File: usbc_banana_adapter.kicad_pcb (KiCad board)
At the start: 2 copper layers, 32 x 25 mm, 26 parts, among them P1 UJ20-C-V-C-3-SMT-TR, SW1 DSHP02TJGER, U1 TPS25810RVCR, U3 TPS2514DBVR

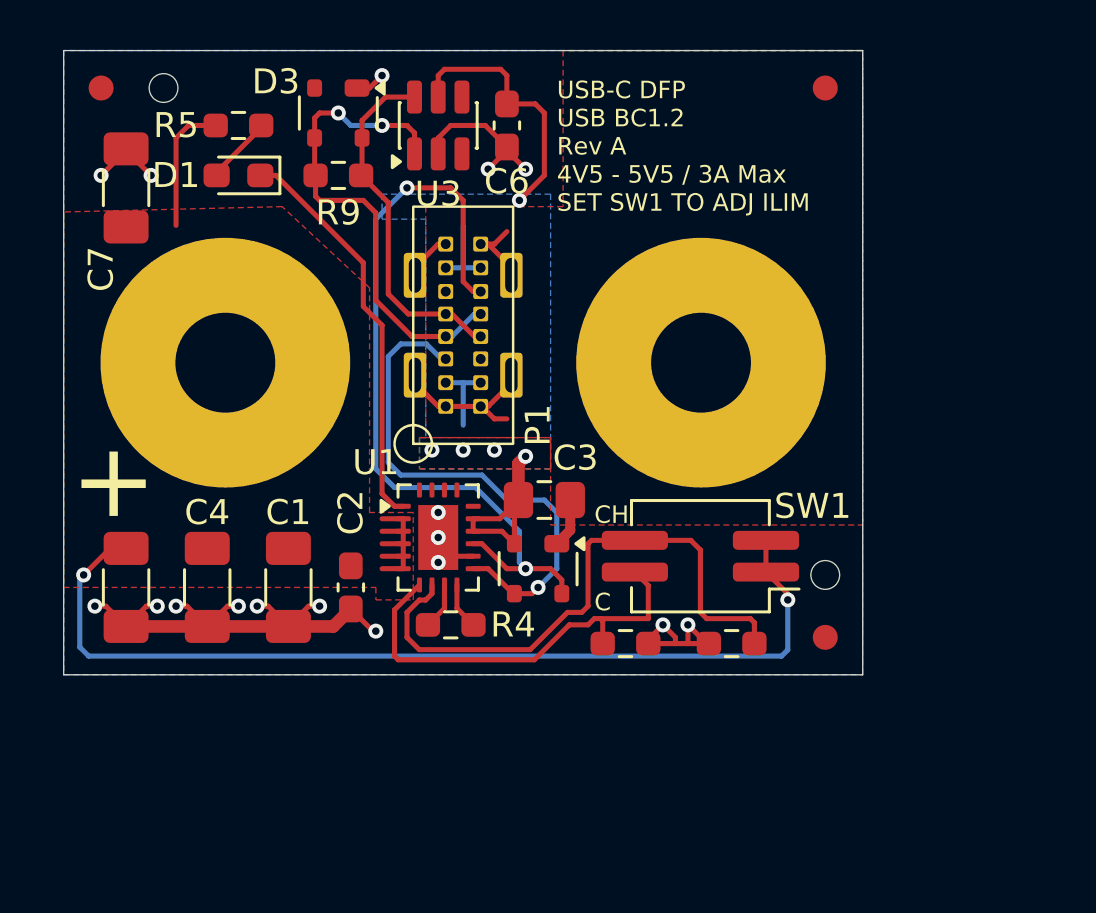
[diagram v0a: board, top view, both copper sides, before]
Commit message: swap banana
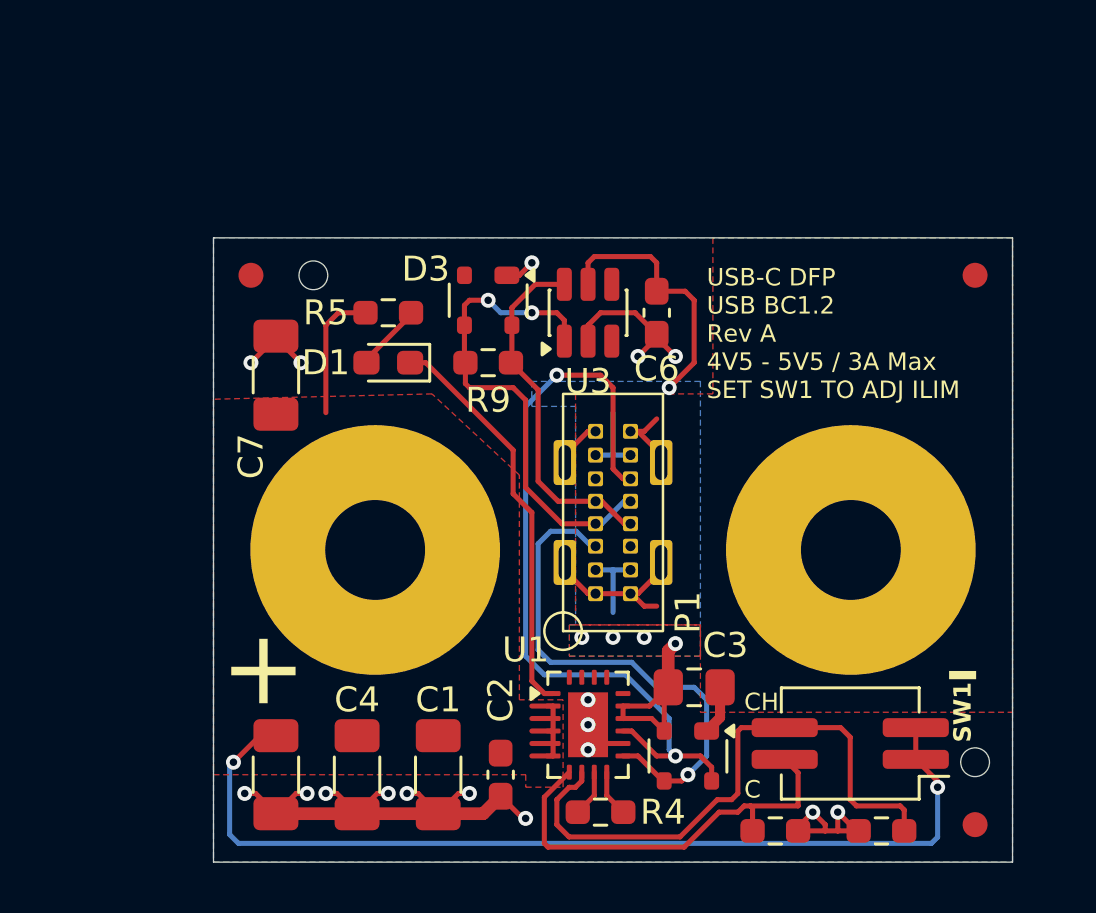
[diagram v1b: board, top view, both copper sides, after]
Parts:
- moved C1 9.60 mm to (109.0, 96.5)
- moved C2 9.60 mm to (111.5, 96.5)
- moved C3 9.60 mm to (119.2, 93.0)
- moved C4 9.60 mm to (105.8, 96.5)
- moved C5 9.60 mm to (102.5, 96.5)
- moved C6 9.60 mm to (117.8, 78.0)
- moved C7 9.60 mm to (102.5, 80.5)
- moved D1 9.60 mm to (107.0, 80.0)
- moved D3 9.60 mm to (111.0, 77.5)
- moved D4 9.60 mm to (119.0, 95.8)
- moved FID1 9.60 mm to (130.5, 76.5)
- moved FID2 9.60 mm to (101.5, 76.5)
- moved FID3 9.60 mm to (130.5, 98.5)
- moved H1 9.60 mm to (106.5, 87.5)
- moved H2 9.60 mm to (125.5, 87.5)
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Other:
- board text added: "-"
